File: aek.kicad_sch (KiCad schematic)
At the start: 243 parts, among them J1 Conn_01x04_MountingPin, SW1 SW_Push, U1 ATmega32U4-MU, Y1 16MHz

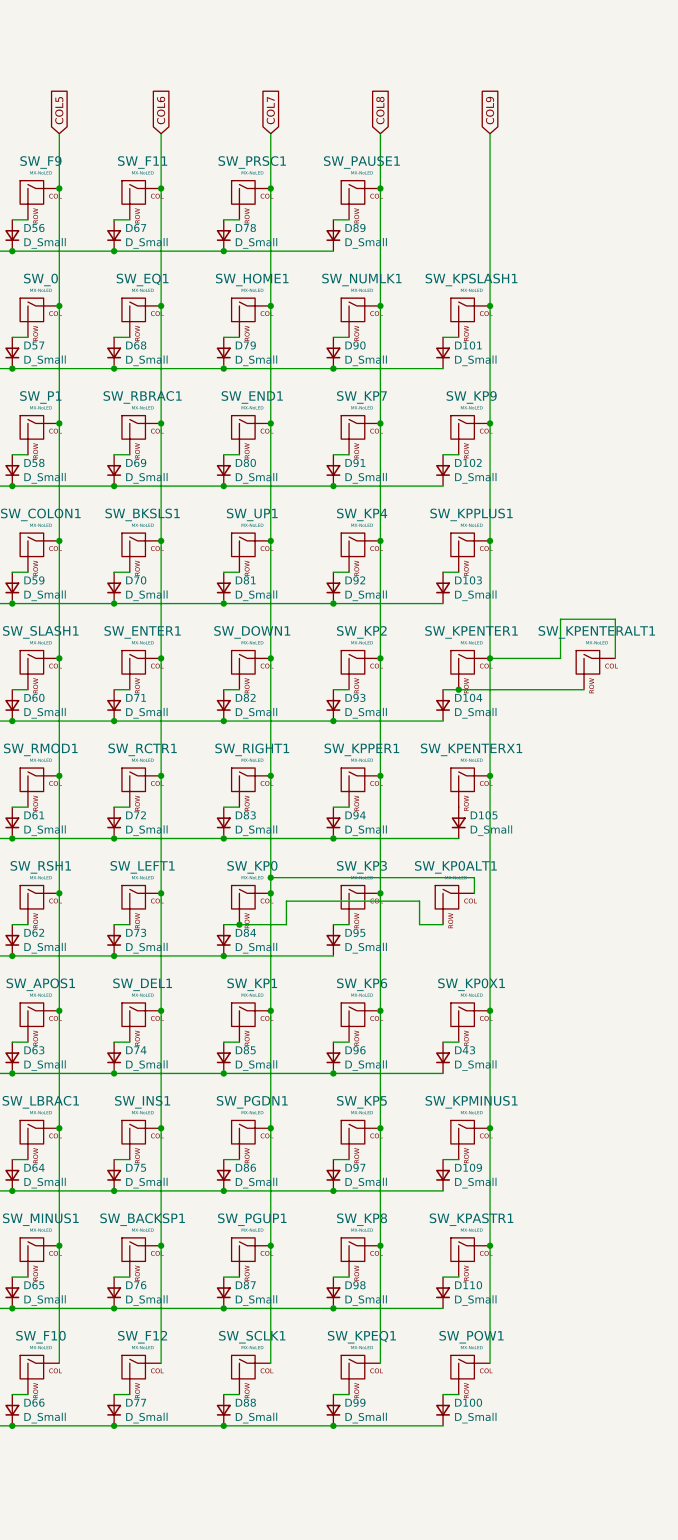
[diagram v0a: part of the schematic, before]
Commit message: ssk branch
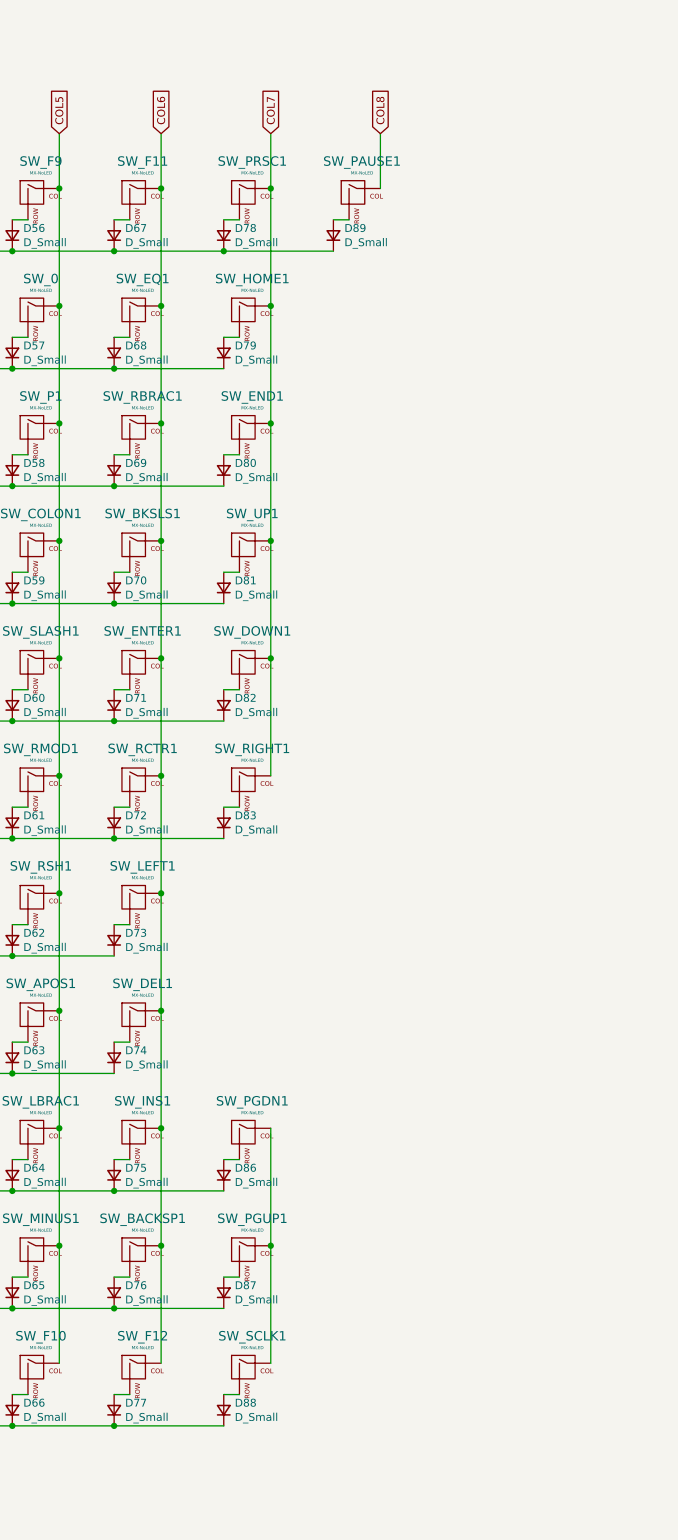
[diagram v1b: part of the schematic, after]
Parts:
- removed D100, D101, D102, D103, D104, D105, D109, D110, D43, D84, D85, D90, D91, D92, D93, D94, D95, D96, D97, D98, D99: D_Small, Diode_SMD:D_SOD-123, symbol Device:D_Small
- removed SW_KP0, SW_KPENTER1: MX-NoLED, MX_Alps_Hybrid:MX-2U-ReversedStabilizers-NoLED, symbol MX_Alps_Hybrid:MX-NoLED
- removed SW_KP0ALT1, SW_KP0X1, SW_KP1, SW_KP2, SW_KP3, SW_KP4, SW_KP5, SW_KP6, SW_KP7, SW_KP8, SW_KP9, SW_KPASTR1, SW_KPENTERALT1, SW_KPENTERX1, SW_KPEQ1, SW_KPMINUS1, SW_KPPER1, SW_KPPLUS1, SW_KPSLASH1, SW_NUMLK1, SW_POW1: MX-NoLED, MX_Alps_Hybrid:MX-1U-NoLED, symbol MX_Alps_Hybrid:MX-NoLED
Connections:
- net COL7: no longer SW_PGDN1.1 (COL), SW_PGUP1.1 (COL), SW_SCLK1.1 (COL)
- new net: SW_PGDN1.1 (COL), SW_PGUP1.1 (COL), SW_SCLK1.1 (COL)
